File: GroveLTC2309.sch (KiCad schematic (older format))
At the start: 9 parts, among them P1 CONN_4_GROVE, P2 CONN_4_GROVE, P3 CONN_4_GROVE, P4 CONN_4_GROVE, P5 CONN_4_GROVE, P6 CONN_4_GROVE, P7 CONN_4_GROVE, P8 CONN_4_GROVE, P9 CONN_4_GROVE

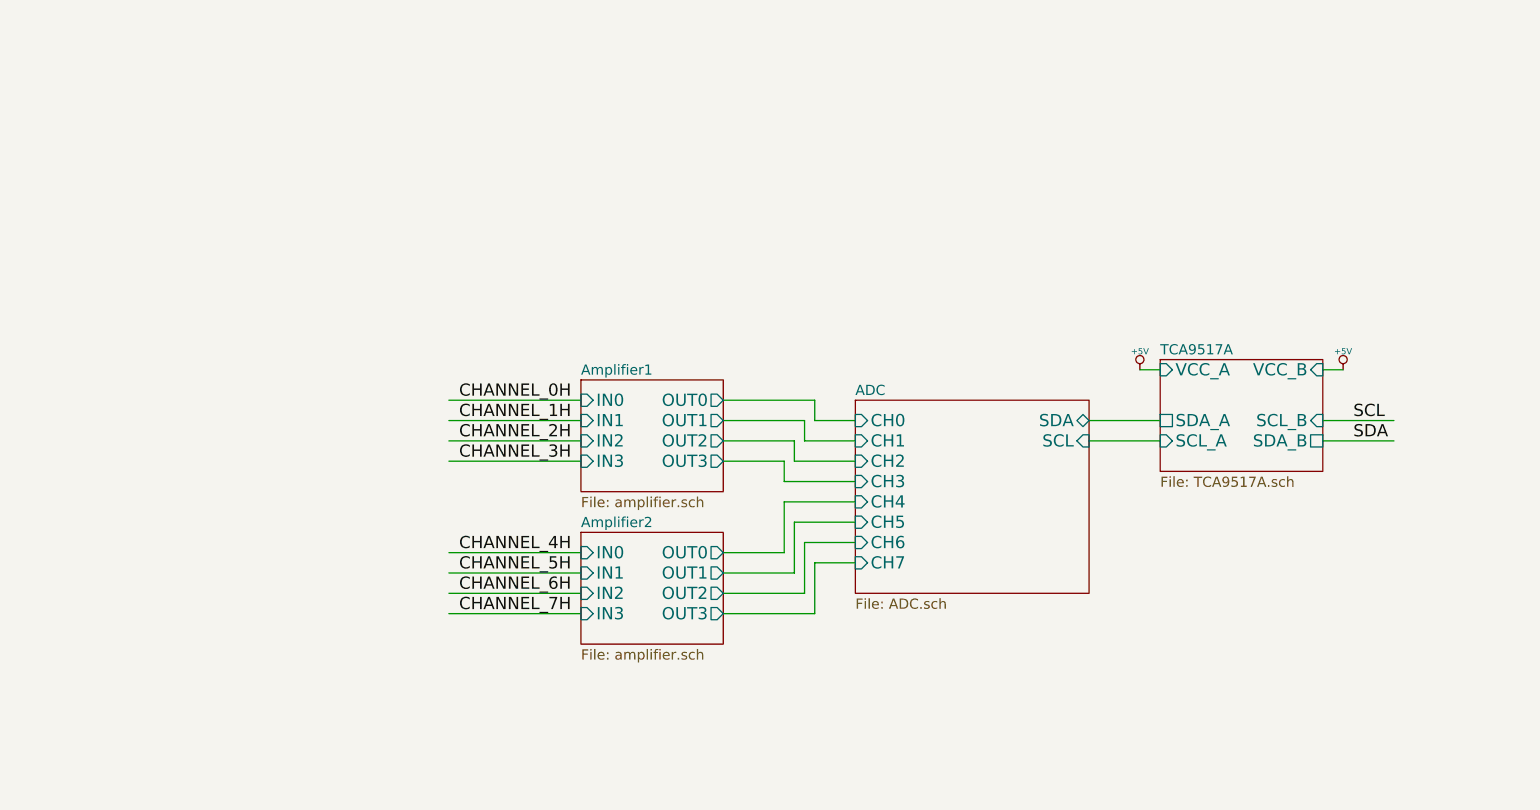
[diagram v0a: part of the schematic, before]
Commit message: version change to 2, first trial for layout revue
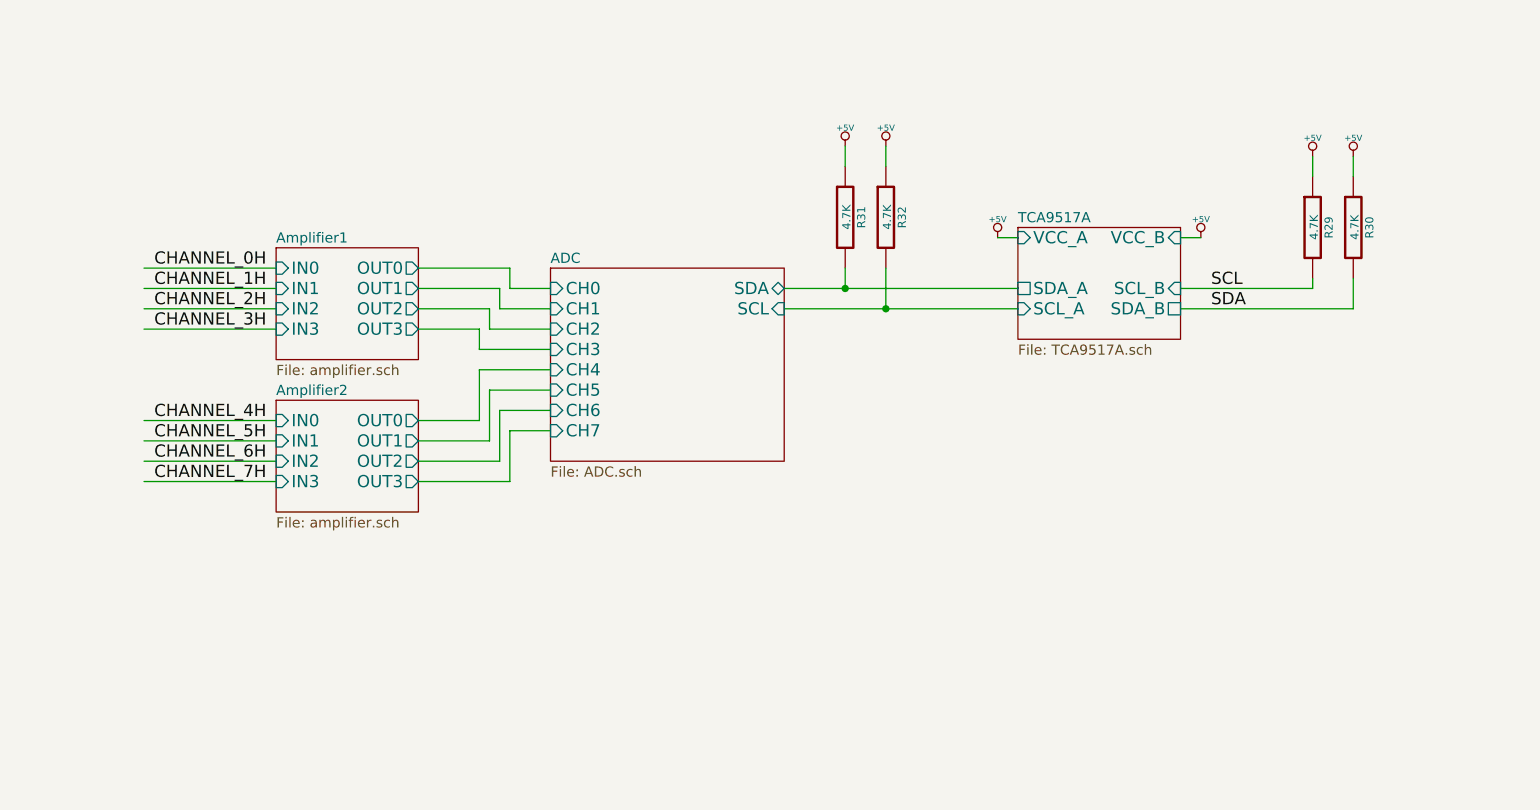
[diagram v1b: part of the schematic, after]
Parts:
- added R29, R30, R31, R32: 4.7K, ~, symbol R
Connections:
- wire segments 69 -> 77
